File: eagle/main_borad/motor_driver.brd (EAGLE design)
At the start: 47.9 x 36.5 mm, 17 parts, among them IC1 MEGA8-AI

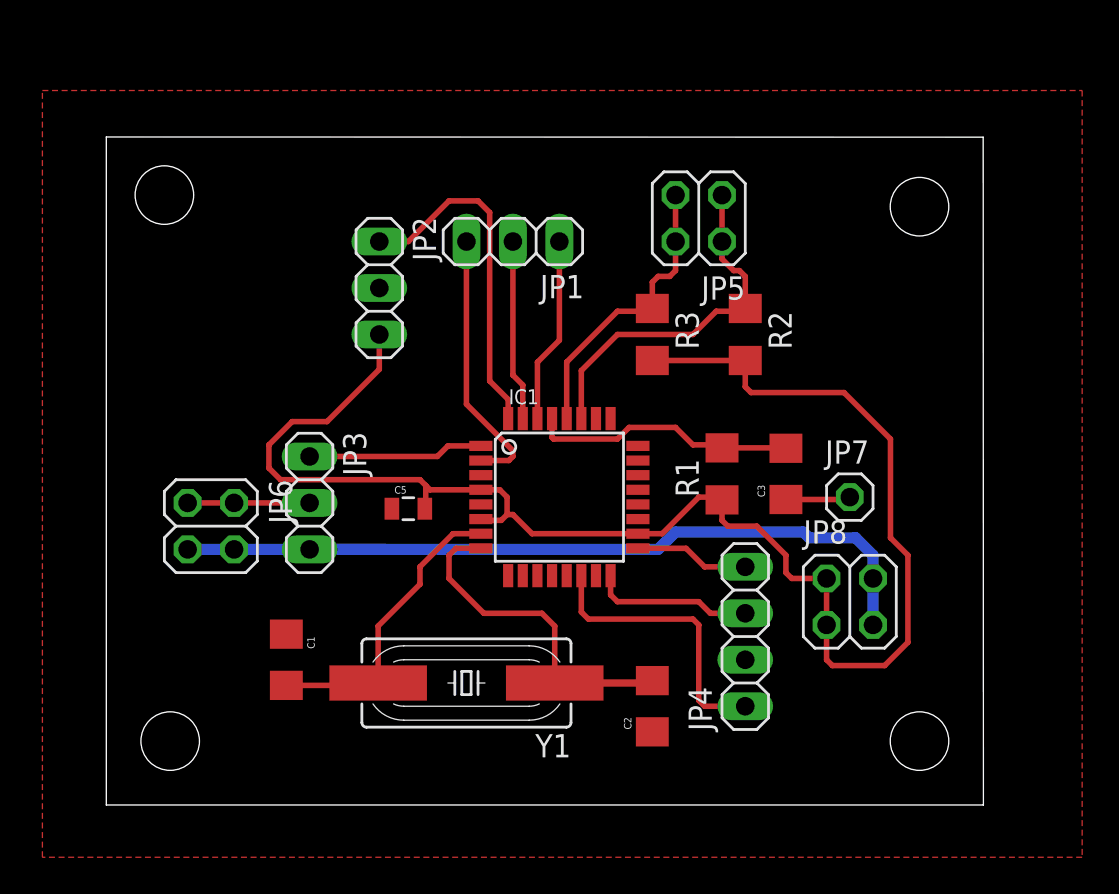
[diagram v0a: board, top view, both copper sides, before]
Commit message: Bugs
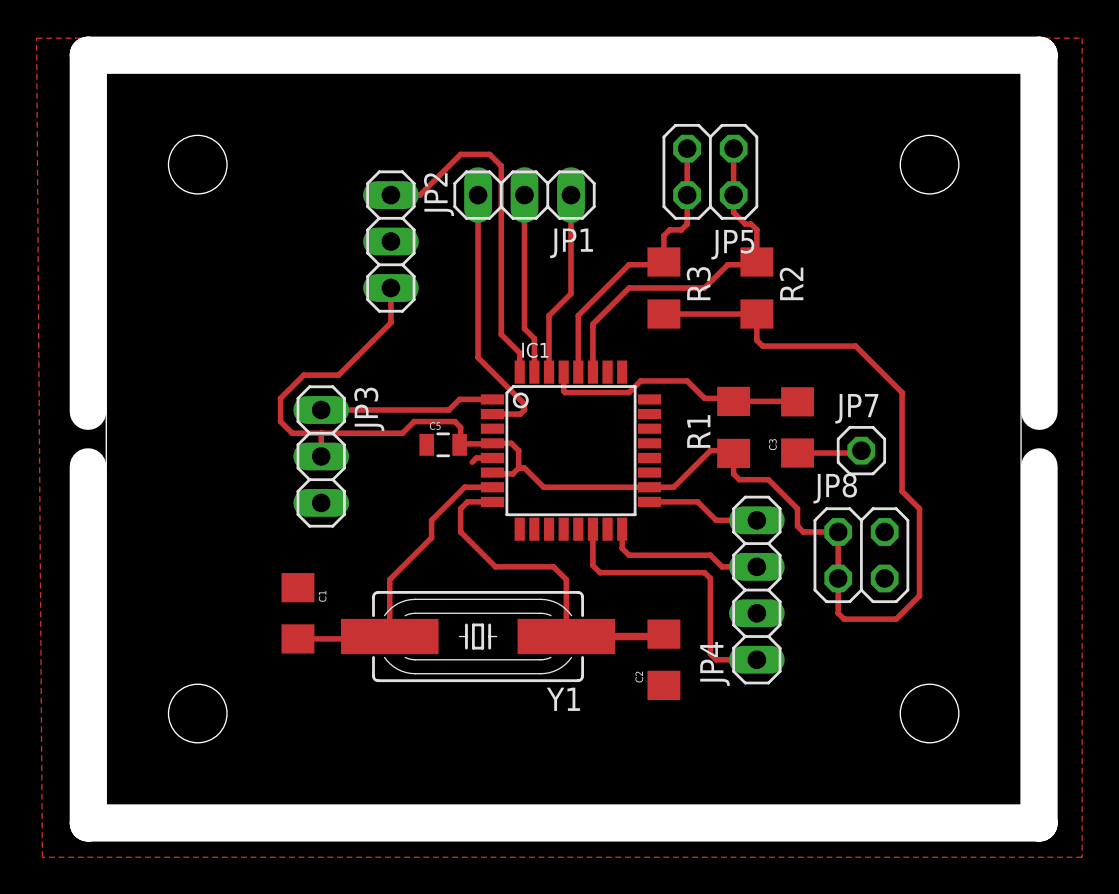
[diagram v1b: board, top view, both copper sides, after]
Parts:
- removed JP6: (no value), pinhead:2X02
- C1, C2: value 220pF -> 22pF
- moved C5 3.98 mm to (18.4, 19.7)
- moved JP4 2.62 mm to (35.6, 11.7)
- moved JP5 2.62 mm to (33.0, 34.6)
- moved R2 2.62 mm to (35.6, 28.3)
- moved C2 2.62 mm to (30.5, 7.94)
- moved R3 2.62 mm to (30.5, 28.3)
- moved Y1 2.62 mm to (20.3, 9.21)
- moved C1 2.62 mm to (10.5, 10.5)
- moved JP2 2.62 mm to (15.6, 30.8)
- moved JP3 2.62 mm to (11.7, 19.1)
- moved C3 2.62 mm to (37.8, 20.6)
- moved IC1 2.62 mm to (25.4, 19.4)
- moved JP1 2.62 mm to (22.9, 33.3)
- moved JP7 2.62 mm to (41.3, 19.4)
- moved JP8 2.62 mm to (41.3, 13.7)
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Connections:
- net GND: no longer JP6.3, JP6.4
- net VCC: no longer JP6.1, JP6.2
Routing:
- net GND: track 46.3 -> 1.20 mm
- net VCC: track 93.6 -> 88.0 mm
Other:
- board size 47.9 x 36.5 mm -> 52 x 42 mm
